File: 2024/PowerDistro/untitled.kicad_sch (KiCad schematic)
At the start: 45 parts, among them J18 Conn_01x02_Pin

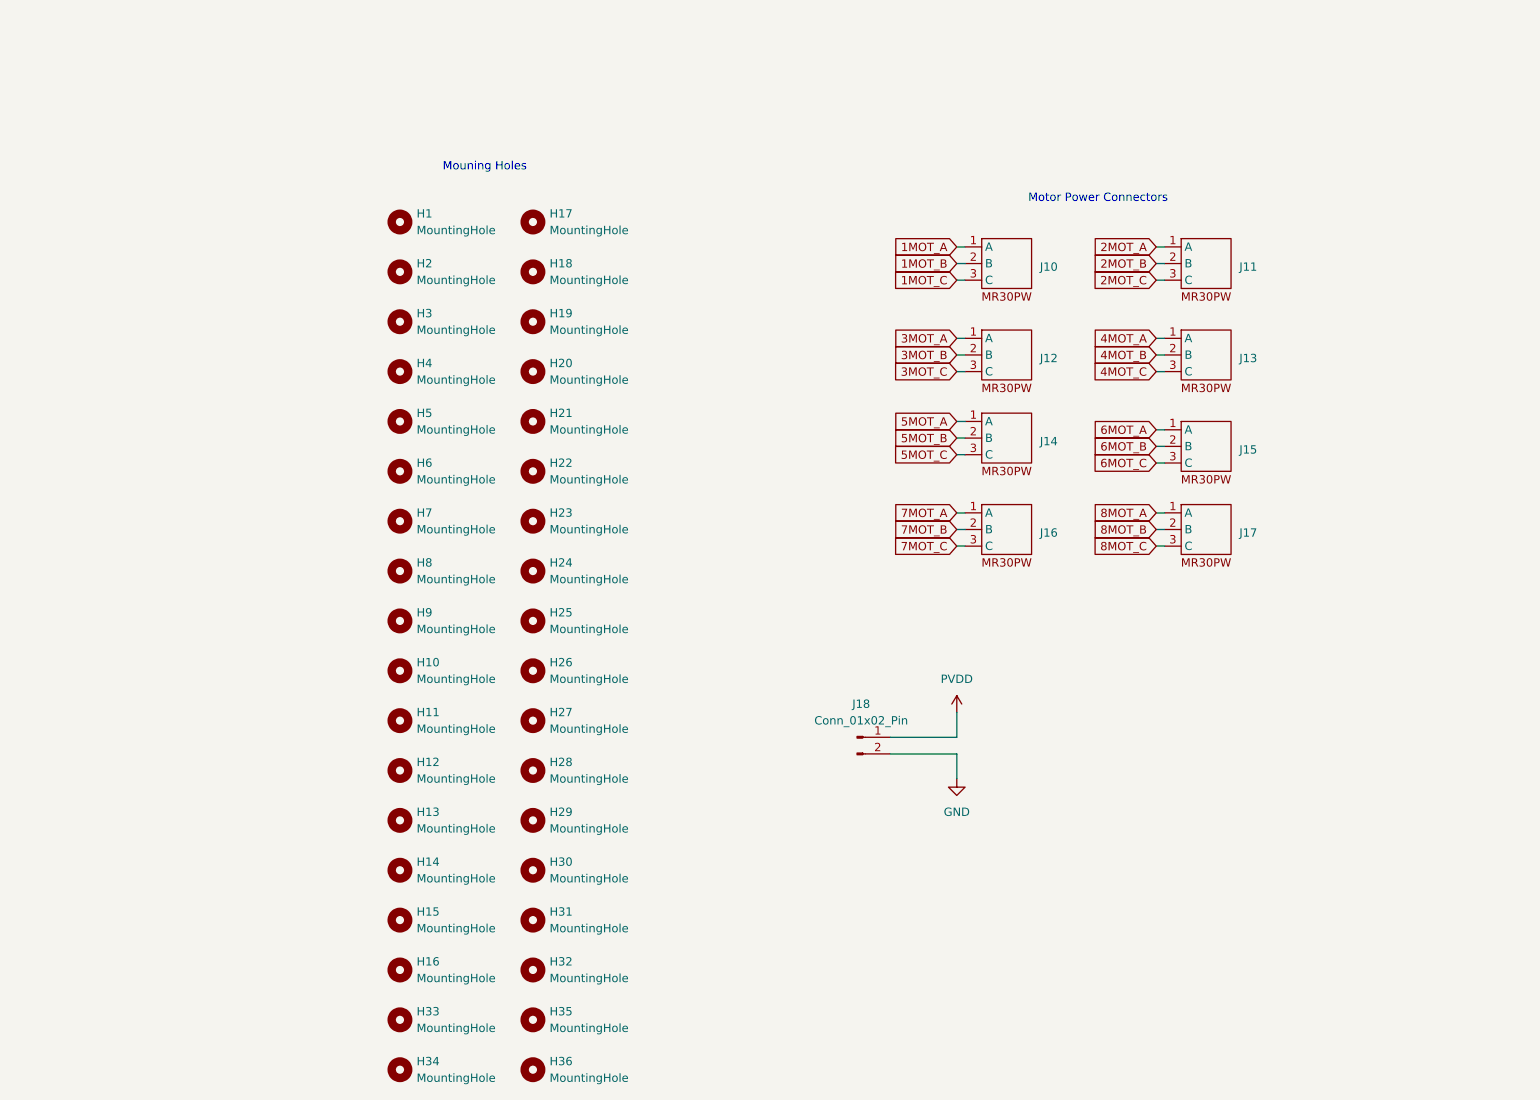
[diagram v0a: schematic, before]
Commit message: Changed Everything
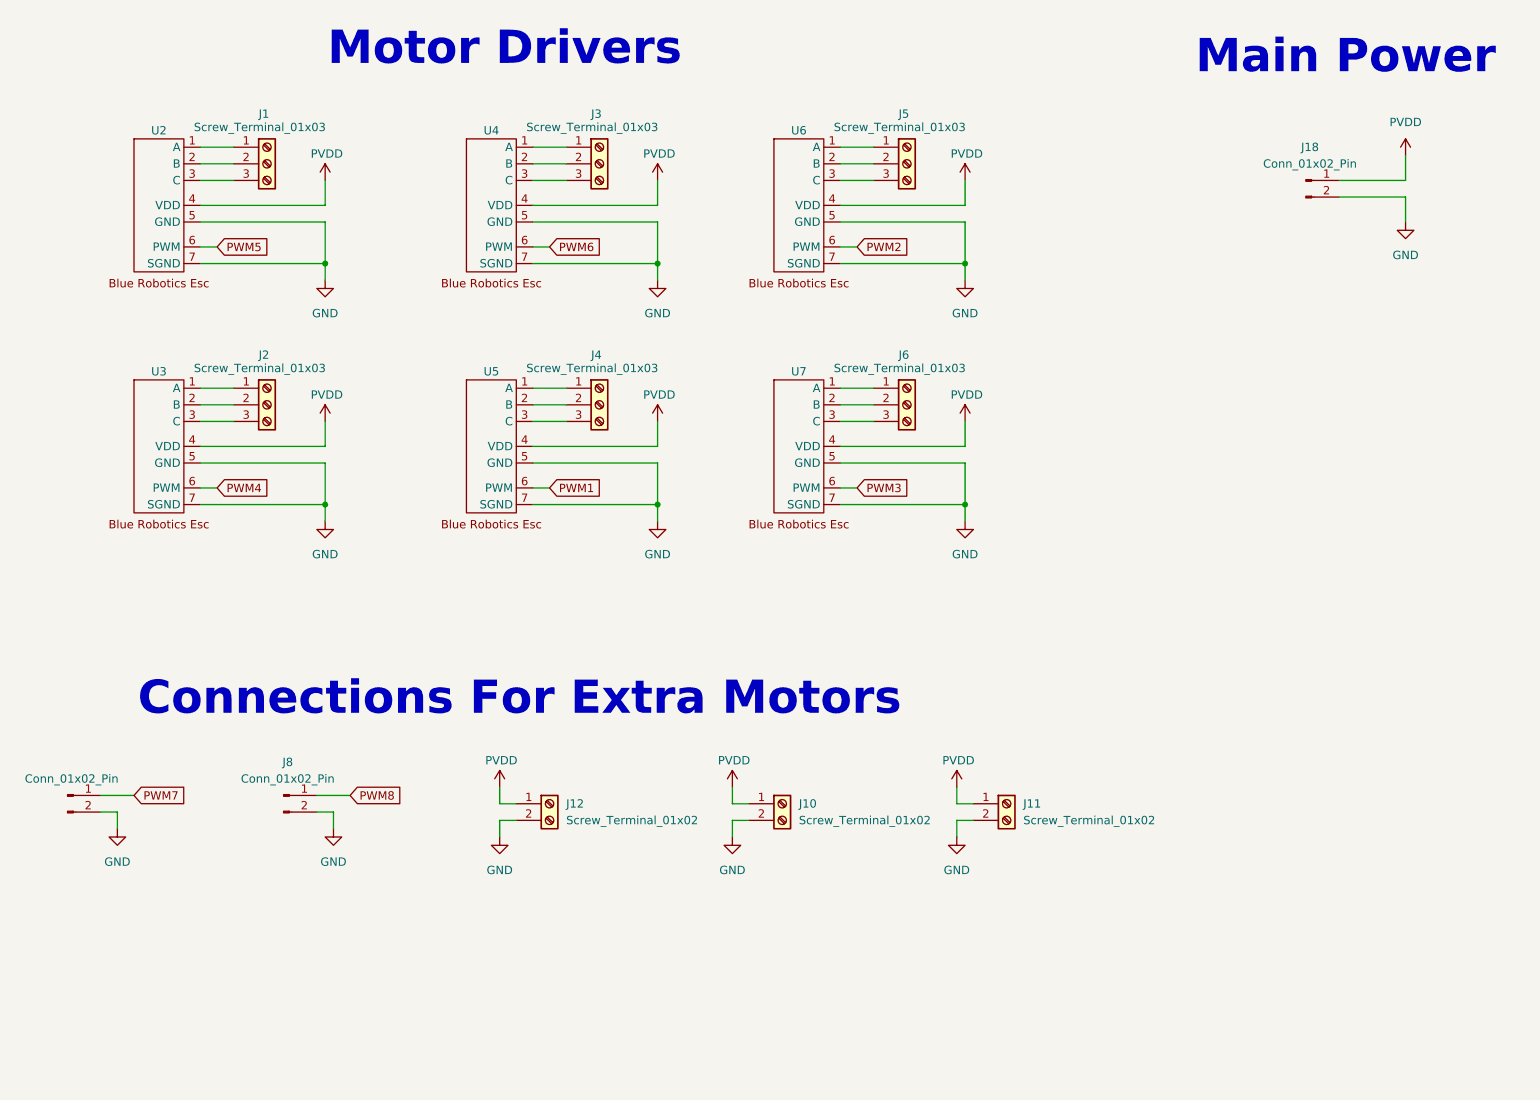
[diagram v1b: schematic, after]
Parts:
- removed H1, H10, H11, H12, H13, H14, H15, H16, H17, H18, H19, H2, H20, H21, H22, H23, H24, H25, H26, H27, H28, H29, H3, H30, H31, H32, H4, H5, H6, H7, H8, H9: MountingHole, MountingHole:MountingHole_2.7mm_M2.5_ISO7380, symbol Mechanical:MountingHole
- removed H33, H34, H35, H36: MountingHole, MountingHole:MountingHole_4.3mm_M4_ISO7380, symbol Mechanical:MountingHole
- removed J10, J11, J12, J13, J14, J15, J16, J17: ~, PowerDistroFootprints:MR30PB, symbol PowerDistro:MR30PW-M
- added J1, J2, J3, J4, J5, J6: Screw_Terminal_01x03, PowerDistroFootprints:691311500103, symbol Connector:Screw_Terminal_01x03
- added J10, J11, J12: Screw_Terminal_01x02, PowerDistroFootprints:691311500102, symbol Connector:Screw_Terminal_01x02
- added J7, J8: Conn_01x02_Pin, Connector_PinHeader_2.54mm:PinHeader_1x02_P2.54mm_Vertical, symbol Connector:Conn_01x02_Pin
- added U2, U3, U4, U5, U6, U7: ~, PowerDistroFootprints:BlueRoboticsESC, symbol PowerDistro:BlueRoboticsESC
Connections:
- net GND: now also J10.2 (Pin_2), J11.2 (Pin_2), J12.2 (Pin_2), J7.2 (Pin_2), J8.2 (Pin_2), U2.5 (GND), U2.7 (SGND), U3.5 (GND), U3.7 (SGND), U4.5 (GND), U4.7 (SGND), U5.5 (GND), U5.7 (SGND), U6.5 (GND), U6.7 (SGND), U7.5 (GND), U7.7 (SGND)
- net PVDD: now also J10.1 (Pin_1), J11.1 (Pin_1), J12.1 (Pin_1), U2.4 (VDD), U3.4 (VDD), U4.4 (VDD), U5.4 (VDD), U6.4 (VDD), U7.4 (VDD)
- new net: J3.1 (Pin_1), U4.1 (A)
- new net: J3.2 (Pin_2), U4.2 (B)
- new net: J3.3 (Pin_3), U4.3 (C)
- new net: J2.1 (Pin_1), U3.1 (A)
- new net: J2.2 (Pin_2), U3.2 (B)
- new net: J2.3 (Pin_3), U3.3 (C)
- new net: J6.1 (Pin_1), U7.1 (A)
- new net: J6.2 (Pin_2), U7.2 (B)
- new net: J6.3 (Pin_3), U7.3 (C)
- new net: J1.1 (Pin_1), U2.1 (A)
- new net: J1.2 (Pin_2), U2.2 (B)
- new net: J1.3 (Pin_3), U2.3 (C)
- new net: J5.1 (Pin_1), U6.1 (A)
- new net: J5.2 (Pin_2), U6.2 (B)
- new net: J5.3 (Pin_3), U6.3 (C)
- new net: J4.1 (Pin_1), U5.1 (A)
- new net: J4.2 (Pin_2), U5.2 (B)
- new net: J4.3 (Pin_3), U5.3 (C)
- new net PWM1: U5.6 (PWM)
- new net PWM2: U6.6 (PWM)
- new net PWM3: U7.6 (PWM)
- new net PWM4: U3.6 (PWM)
- new net PWM5: U2.6 (PWM)
- new net PWM6: U4.6 (PWM)
- new net PWM7: J7.1 (Pin_1)
- new net PWM8: J8.1 (Pin_1)
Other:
- note added: "Connections For Extra Motors"
- note added: "Main Power"
- note added: "Motor Drivers"
- note removed: "Motor Power Connectors"
- note removed: "Mouning Holes"
- moved on the sheet: J18
